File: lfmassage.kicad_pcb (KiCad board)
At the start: 2 copper layers, 1 part, among them IC1 EFM8BB31F16G-D-QFN24

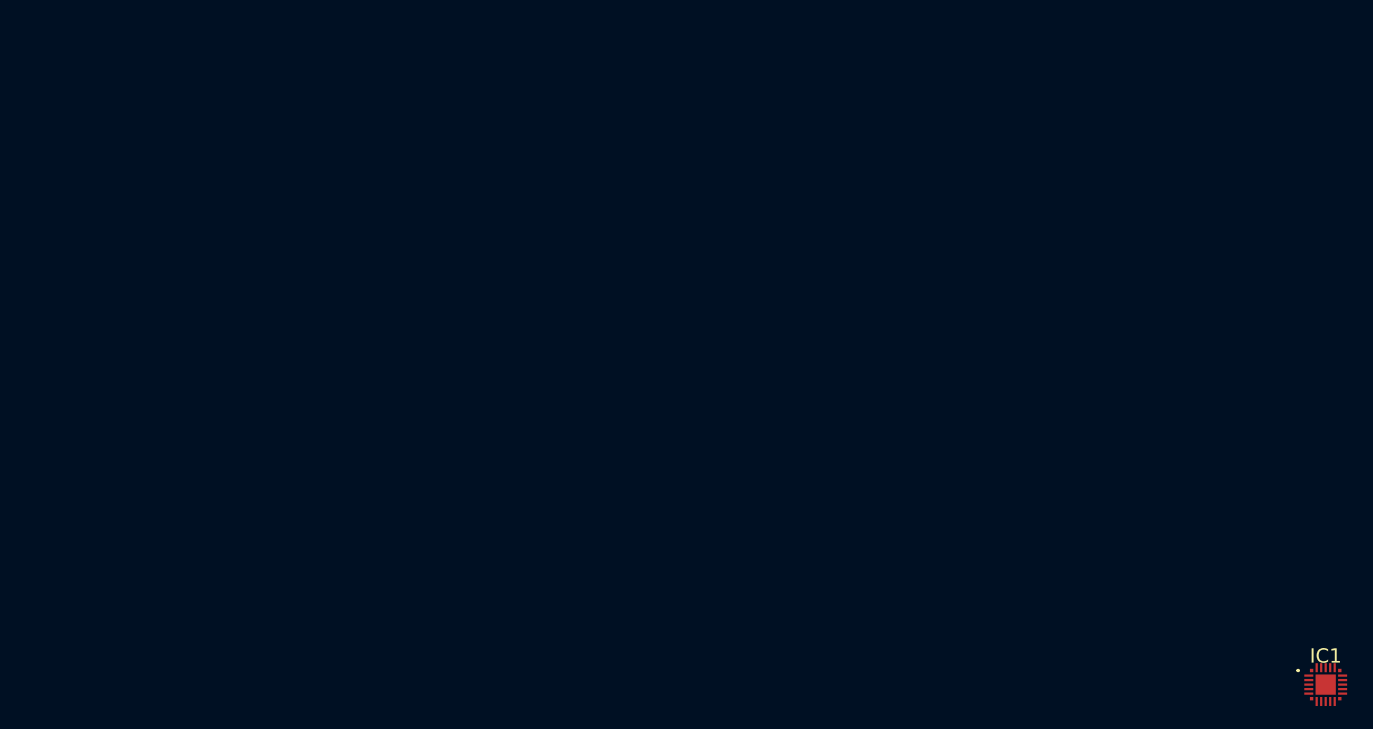
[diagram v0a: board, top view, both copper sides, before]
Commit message: 2022-07-11
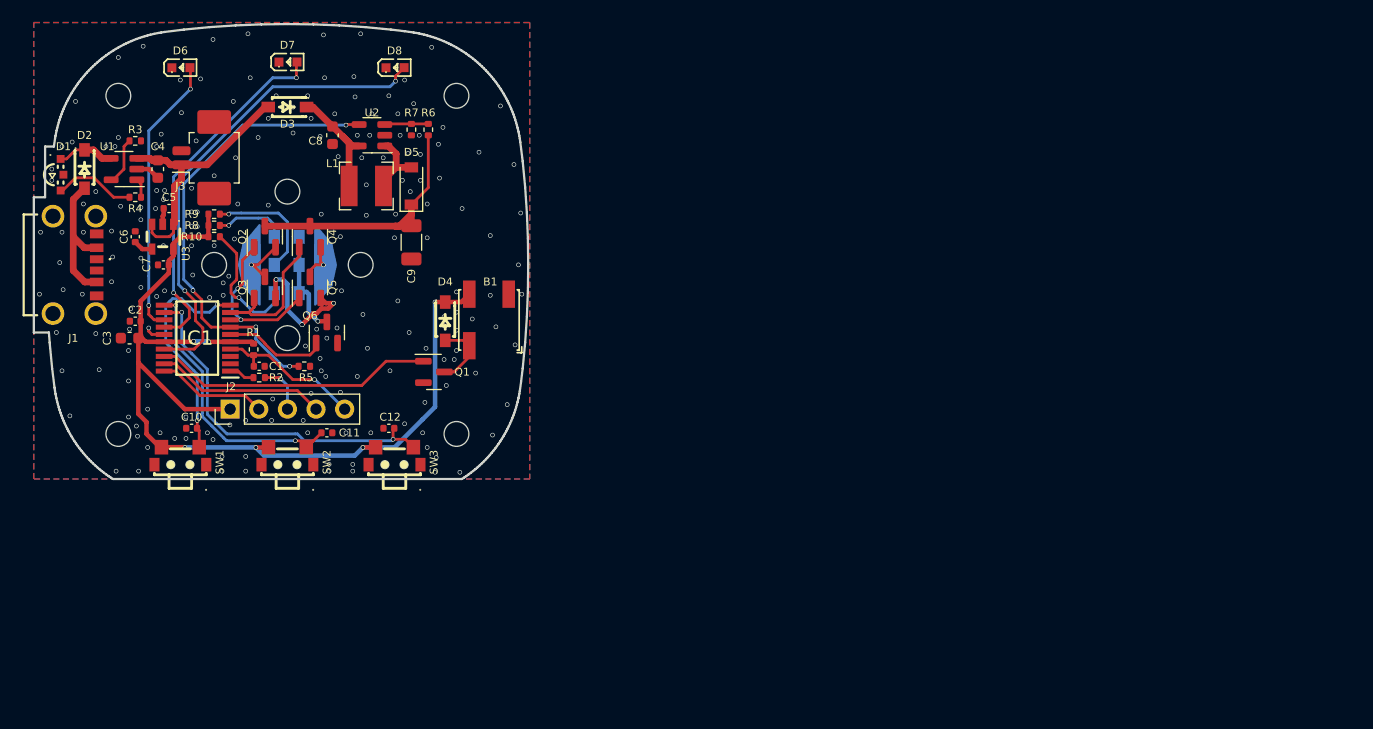
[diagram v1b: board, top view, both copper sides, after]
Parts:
- added B1: MLT-5030, MLT-5030:MLT-5030, F.Cu at (60.5, 46.5)
- added C1: 100nF, Capacitor_SMD:C_0402_1005Metric, F.Cu at (40.0, 50.5)
- added C10: 100nF, Capacitor_SMD:C_0402_1005Metric, F.Cu at (34.0, 56.0)
- added C11: 100nF, Capacitor_SMD:C_0402_1005Metric, F.Cu at (46.0, 56.4)
- added C12: 100nF, Capacitor_SMD:C_0402_1005Metric, F.Cu at (51.5, 56.0)
- added C2: 100nF, Capacitor_SMD:C_0402_1005Metric, F.Cu at (29.0, 46.5)
- added C3: 10uF, Capacitor_SMD:C_0603_1608Metric, F.Cu at (28.5, 48.0)
- added C4: 10uF, Capacitor_SMD:C_0603_1608Metric, F.Cu at (31.0, 33.0)
- added C5: 1uF, Capacitor_SMD:C_0402_1005Metric, F.Cu at (32.0, 36.5)
- added C6: 10nF, Capacitor_SMD:C_0402_1005Metric, F.Cu at (29.0, 39.0)
- added C7: 1uF, Capacitor_SMD:C_0402_1005Metric, F.Cu at (31.5, 41.5)
- added C8: 10uF, Capacitor_SMD:C_0603_1608Metric, F.Cu at (46.5, 30.0)
- added C9: 10uF, Capacitor_SMD:C_1206_3216Metric, F.Cu at (53.5, 39.5)
- added D1: MHS110KECT, MHS110KECT:LED-ARRAY-SMD_3P-L3.00-W1.50-R-RD, F.Cu at (22.0, 33.5)
- added D10: IR LED, XL-1608UWC-04:LED0805-RD, B.Cu at (42.5, 41.5)
- added D11: RED LED, XL-1608UWC-04:LED0805-RD, B.Cu at (42.5, 44.0)
- added D2: 1N4148W-7-F, 1N4148W-7-F:SOD-123_L2.7-W1.6-LS3.7-RD-1, F.Cu at (24.5, 33.0)
- added D3: 1N4148W-7-F, 1N4148W-7-F:SOD-123_L2.7-W1.6-LS3.7-RD-1, F.Cu at (42.5, 27.5)
- added D4: 1N4148W-7-F, 1N4148W-7-F:SOD-123_L2.7-W1.6-LS3.7-RD-1, F.Cu at (56.5, 46.5)
- added D5: DSK34, Diode_SMD:D_SOD-123, F.Cu at (53.5, 34.5)
- added D6: LED, XL-1608UWC-04:XL-1608UWC-04, F.Cu at (33.0, 24.0)
- added D7: LED, XL-1608UWC-04:XL-1608UWC-04, F.Cu at (42.5, 23.5)
- added D8: LED, XL-1608UWC-04:XL-1608UWC-04, F.Cu at (52.0, 24.0)
- added D9: RED LED, XL-1608UWC-04:LED0805-RD, B.Cu at (42.5, 39.0)
- added E1: SparkGap, Electrode:Electrode, B.Cu at (42.5, 41.5)
- added J1: USB4125-GF-A-0190, USB4125-GF-A-0190:USB4125GFA0190, F.Cu at (22.5, 41.5)
- added J2: SWD, Connector_PinHeader_2.54mm:PinHeader_1x05_P2.54mm_Vertical, F.Cu at (37.4, 54.3)
- added J3: 53261-0271, Connector_Molex:Molex_PicoBlade_53261-0271_1x02-1MP_P1.25mm_Horizontal, F.Cu at (35.5, 32.0)
- added L1: 4.7uH, Inductor_SMD:L_Bourns-SRN4018, F.Cu at (49.5, 34.5)
- added M1: MountingHole, MountingHole:MountingHole_2.2mm_M2, F.Cu at (27.5, 56.5)
- added M2: MountingHole, MountingHole:MountingHole_2.2mm_M2, F.Cu at (57.5, 56.5)
- added M3: MountingHole, MountingHole:MountingHole_2.2mm_M2, F.Cu at (57.5, 26.5)
- added M4: MountingHole, MountingHole:MountingHole_2.2mm_M2, F.Cu at (27.5, 26.5)
- added M5: MountingHole, MountingHole:MountingHole_2.2mm_M2, F.Cu at (42.5, 48.0)
- added M6: MountingHole, MountingHole:MountingHole_2.2mm_M2, F.Cu at (49.0, 41.5)
- added M7: MountingHole, MountingHole:MountingHole_2.2mm_M2, F.Cu at (42.5, 35.0)
- added M8: MountingHole, MountingHole:MountingHole_2.2mm_M2, F.Cu at (36.0, 41.5)
- added Q1: N-FET, Package_TO_SOT_SMD:SOT-23, F.Cu at (55.5, 51.0)
- added Q2: N-FET, Package_TO_SOT_SMD:SOT-23, F.Cu at (40.5, 39.0)
- added Q3: N-FET, Package_TO_SOT_SMD:SOT-23, F.Cu at (40.5, 43.5)
- added Q4: N-FET, Package_TO_SOT_SMD:SOT-23, F.Cu at (44.5, 39.0)
- added Q5: N-FET, Package_TO_SOT_SMD:SOT-23, F.Cu at (44.5, 43.5)
- added Q6: N-FET, Package_TO_SOT_SMD:SOT-23, F.Cu at (46.0, 47.5)
- added R1: 47k, Resistor_SMD:R_0402_1005Metric, F.Cu at (39.5, 49.0)
- added R10: 100, Resistor_SMD:R_0402_1005Metric, F.Cu at (36.0, 39.0)
- added R2: 47k, Resistor_SMD:R_0402_1005Metric, F.Cu at (40.0, 51.5)
- added R3: 10k, Resistor_SMD:R_0402_1005Metric, F.Cu at (29.0, 30.5)
- added R4: 680, Resistor_SMD:R_0402_1005Metric, F.Cu at (29.0, 35.5)
- added R5: 47k, Resistor_SMD:R_0402_1005Metric, F.Cu at (44.0, 50.5)
- added R6: 180k, Resistor_SMD:R_0402_1005Metric, F.Cu at (55.0, 29.5)
- added R7: 8.2k, Resistor_SMD:R_0402_1005Metric, F.Cu at (53.5, 29.5)
- added R8: 100, Resistor_SMD:R_0402_1005Metric, F.Cu at (36.0, 38.0)
- added R9: 100, Resistor_SMD:R_0402_1005Metric, F.Cu at (36.0, 37.0)
- added SW1: TS24CA, TS24CA:TS24CA, F.Cu at (33.0, 59.5)
- added SW2: TS24CA, TS24CA:TS24CA, F.Cu at (42.5, 59.5)
- added SW3: TS24CA, TS24CA:TS24CA, F.Cu at (52.0, 59.5)
- added U1: MCP73831-2-OT, Package_TO_SOT_SMD:SOT-23-5, F.Cu at (28.0, 33.0)
- added U2: MT3540, Package_TO_SOT_SMD:SOT-23-5, F.Cu at (50.0, 30.0)
- added U3: RS3236-2_8YF5, RS3236-2.8YF5:SOT-23-5_L2.9-W1.6-P0.95-LS2.8-BL, F.Cu at (31.5, 39.0)
- IC1: value EFM8BB31F16G-D-QFN24 -> STM32L010F4P6; footprint EFM8BB31F16G-D-QFN24:EFM8BB31F16GDQFN24 -> STM32L010F4P6:SOP65P640X120-20N
- moved IC1 104.7 mm to (34.5, 48.0), turned to 180 degrees
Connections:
- IC1 pad 1: unconnected-(IC1-Pad1) -> Net-(R2-Pad2)
- IC1 pad 10: unconnected-(IC1-Pad10) -> /PA4
- IC1 pad 11: unconnected-(IC1-Pad11) -> /PA5
- IC1 pad 12: unconnected-(IC1-Pad12) -> /PA6
- IC1 pad 13: unconnected-(IC1-Pad13) -> /PA7
- IC1 pad 14: unconnected-(IC1-Pad14) -> /PB1
- IC1 pad 15: unconnected-(IC1-Pad15) -> GND
- IC1 pad 16: unconnected-(IC1-Pad16) -> +2V8
- IC1 pad 17: unconnected-(IC1-Pad17) -> /PA9
- IC1 pad 18: unconnected-(IC1-Pad18) -> /PA10
- IC1 pad 19: unconnected-(IC1-Pad19) -> /SWDIO
- IC1 pad 20: unconnected-(IC1-Pad20) -> /SWCLK
- IC1 pad 4: unconnected-(IC1-Pad4) -> /nRST
- IC1 pad 5: unconnected-(IC1-Pad5) -> +2V8
- IC1 pad 6: unconnected-(IC1-Pad6) -> /PA0
- IC1 pad 7: unconnected-(IC1-Pad7) -> /PA1
- IC1 pad 8: unconnected-(IC1-Pad8) -> /PA2
- IC1 pad 9: unconnected-(IC1-Pad9) -> /PA3
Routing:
- net +2V8: track 0.00 -> 87.2 mm, vias 0 -> 6
- net /PA9: track 0.00 -> 43.2 mm, vias 0 -> 2
- net /PA1: track 0.00 -> 41.3 mm, vias 0 -> 4
- net /PA6: track 0.00 -> 32.3 mm, vias 0 -> 2
- net /PB1: track 0.00 -> 31.6 mm, vias 0 -> 2
- net /PA7: track 0.00 -> 25.0 mm, vias 0 -> 2
- net /PA10: track 0.00 -> 25.0 mm
- net /PA5: track 0.00 -> 24.8 mm, vias 0 -> 2
- net /HV: track 0.00 -> 23.5 mm
- net /BATT: track 0.00 -> 23.4 mm
- net GND: track 0.00 -> 21.7 mm, vias 0 -> 198
- net /PA4: track 0.00 -> 20.8 mm, vias 0 -> 2
- net /SWDIO: track 0.00 -> 15.1 mm
- net /PA2: track 0.00 -> 14.5 mm, vias 0 -> 2
- net /nRST: track 0.00 -> 13.3 mm, vias 0 -> 1
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- added copper zone on B.Cu, net GND
- added copper zone on F.Cu, net GND
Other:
- board outline added: 43.9 x 40.4 mm
- board text added: ":IR"
- board text added: ":RED"
